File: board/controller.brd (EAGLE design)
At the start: 100 x 100 mm, 70 parts, among them J1 X, J10 FEED_HOLD, J11 PROBE, J12 ERROR, J13 HOLDING, J14 GND, J15 MOTOR_CURRENT, J16 SD_READER, J17 WHEEL, J18 FEED, J19 Z_DISPLAY, J2 Y, J22 +5V, J23 DISPLAY, J24 GND, J25 GND, J26 +5V, J3 Z, J4 A, J5 COOLANT, J6 SPINDLE, J8 RESET, J9 CYCLE_START, U100 SENSOR-IR-THRU

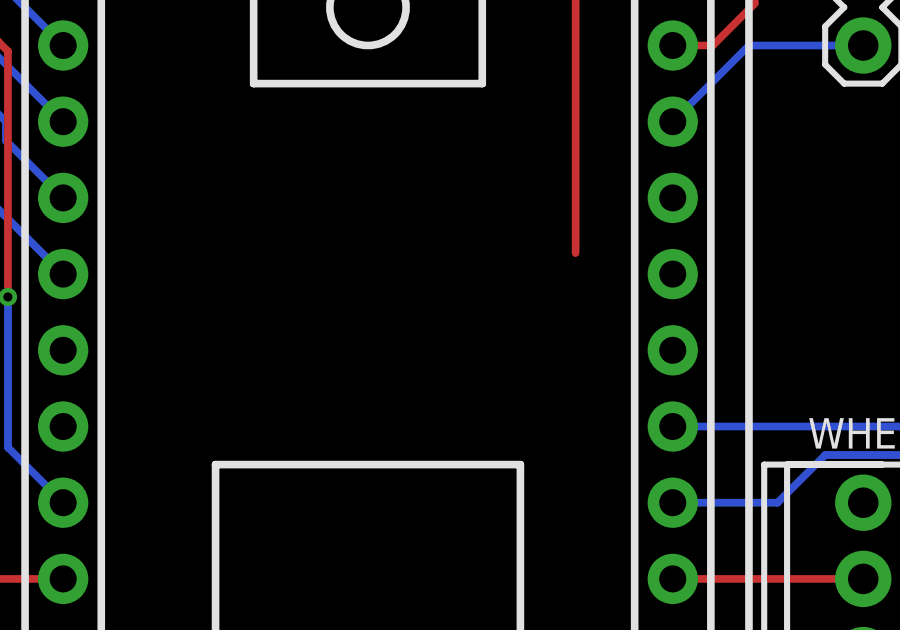
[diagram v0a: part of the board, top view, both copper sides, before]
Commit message: added more documentation
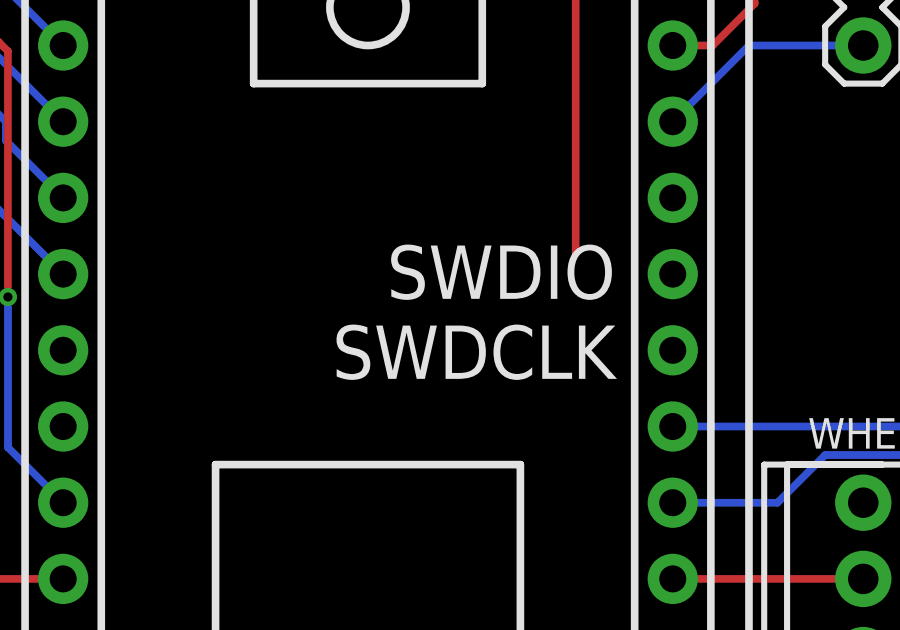
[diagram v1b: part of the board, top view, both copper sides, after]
